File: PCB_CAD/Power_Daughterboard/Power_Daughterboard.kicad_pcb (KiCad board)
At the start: 2 copper layers, 5 parts, among them J1 470531000, J2 CMF2.1111.12

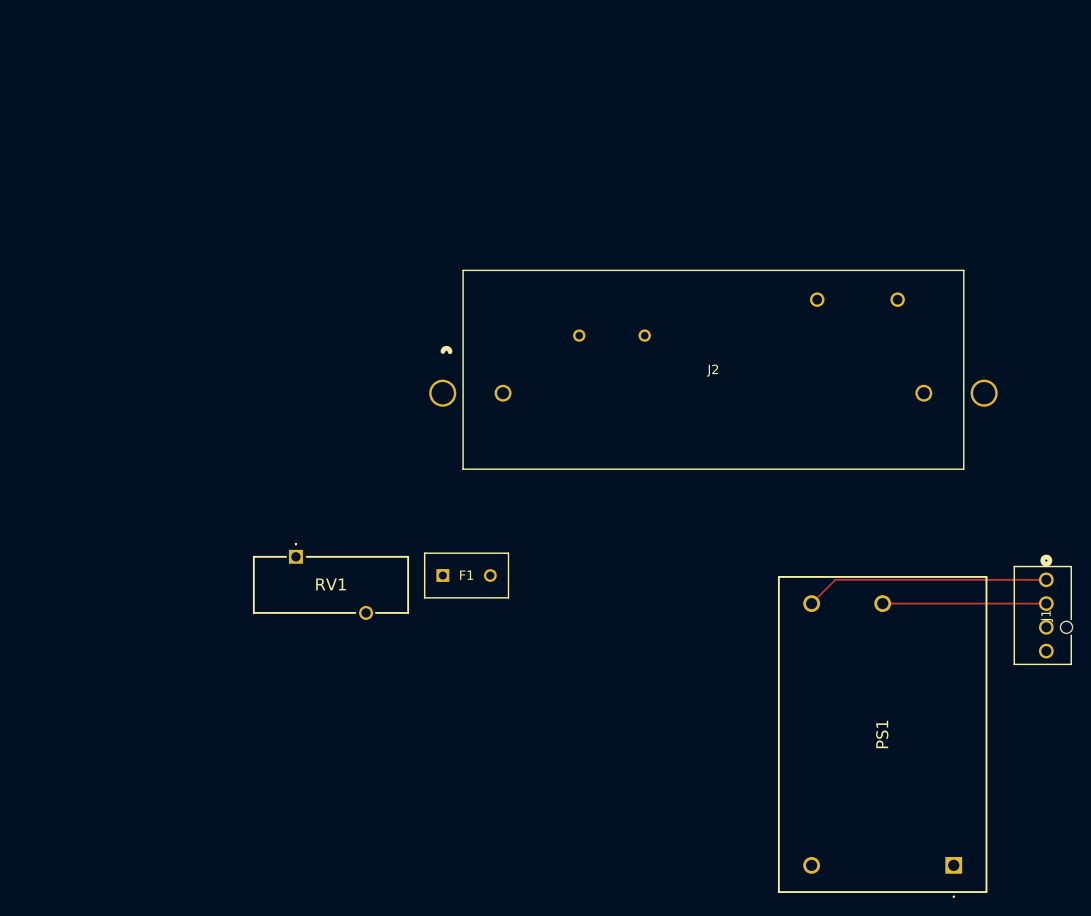
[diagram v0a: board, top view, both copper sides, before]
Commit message: power daughterboard work
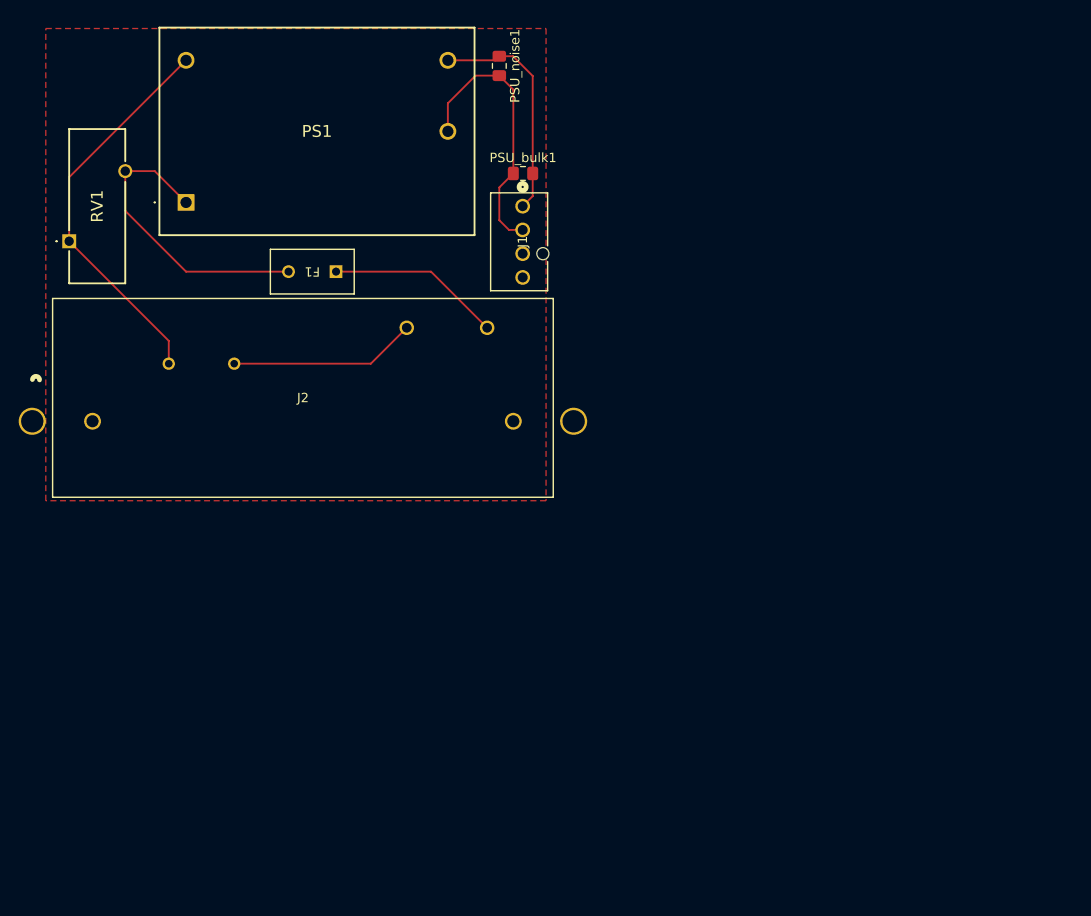
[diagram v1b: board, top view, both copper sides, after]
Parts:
- added PSU_bulk1: 100u, Capacitor_SMD:C_0805_2012Metric_Pad1.18x1.45mm_HandSolder, F.Cu at (169.0, 64.5)
- added PSU_noise1: 0.1u, Capacitor_SMD:C_0805_2012Metric_Pad1.18x1.45mm_HandSolder, F.Cu at (166.5, 53.0)
- moved PS1 108.5 mm to (133.0, 67.6), turned to 0 degrees
- moved J1 68.8 mm to (169.0, 68.0)
- moved J2 44.0 mm to (131.1, 84.8)
- moved RV1 41.6 mm to (120.5, 71.8), turned to 90 degrees
- moved F1 34.4 mm to (149.0, 75.0), turned to 180 degrees
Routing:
- net Net-(PS1-AC2): track 0.00 -> 42.0 mm
- net Net-(PS1-AC1): track 0.00 -> 32.3 mm
- net Net-(J2-Pad2): track 0.00 -> 20.0 mm
- net Net-(F1-Pad1): track 0.00 -> 18.6 mm
- net Net-(PS1-DC+): track 17.5 -> 29.8 mm
- net Net-(PS1-DC-): track 26.2 -> 24.5 mm
- added copper zone on F.Cu, net Net-(PS1-DC+)
